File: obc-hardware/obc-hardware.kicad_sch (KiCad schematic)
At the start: 4 parts

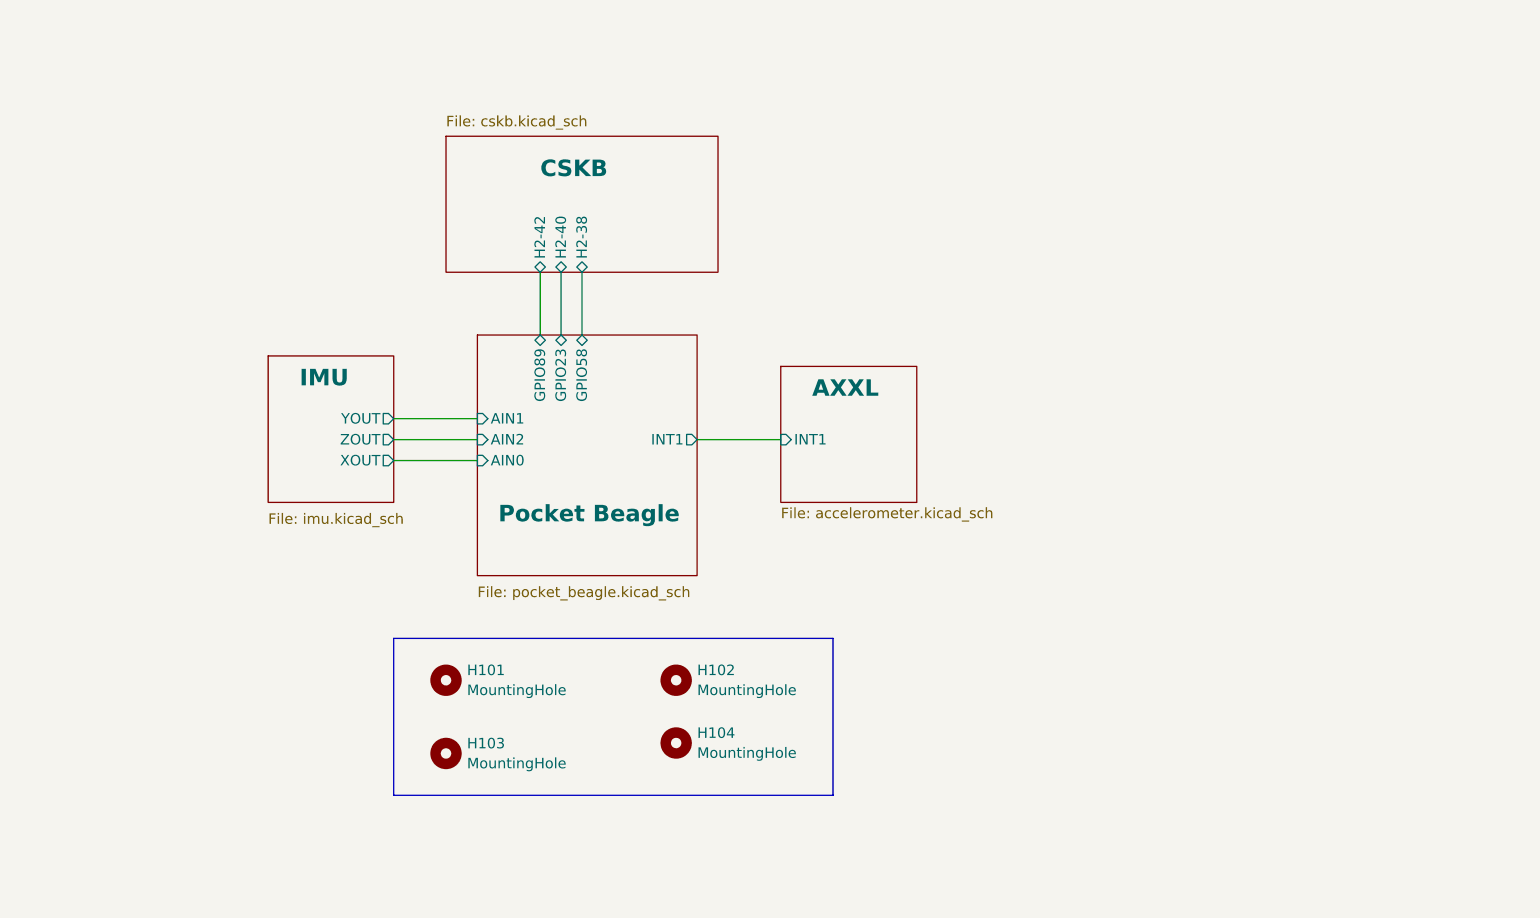
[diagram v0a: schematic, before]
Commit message: added test points
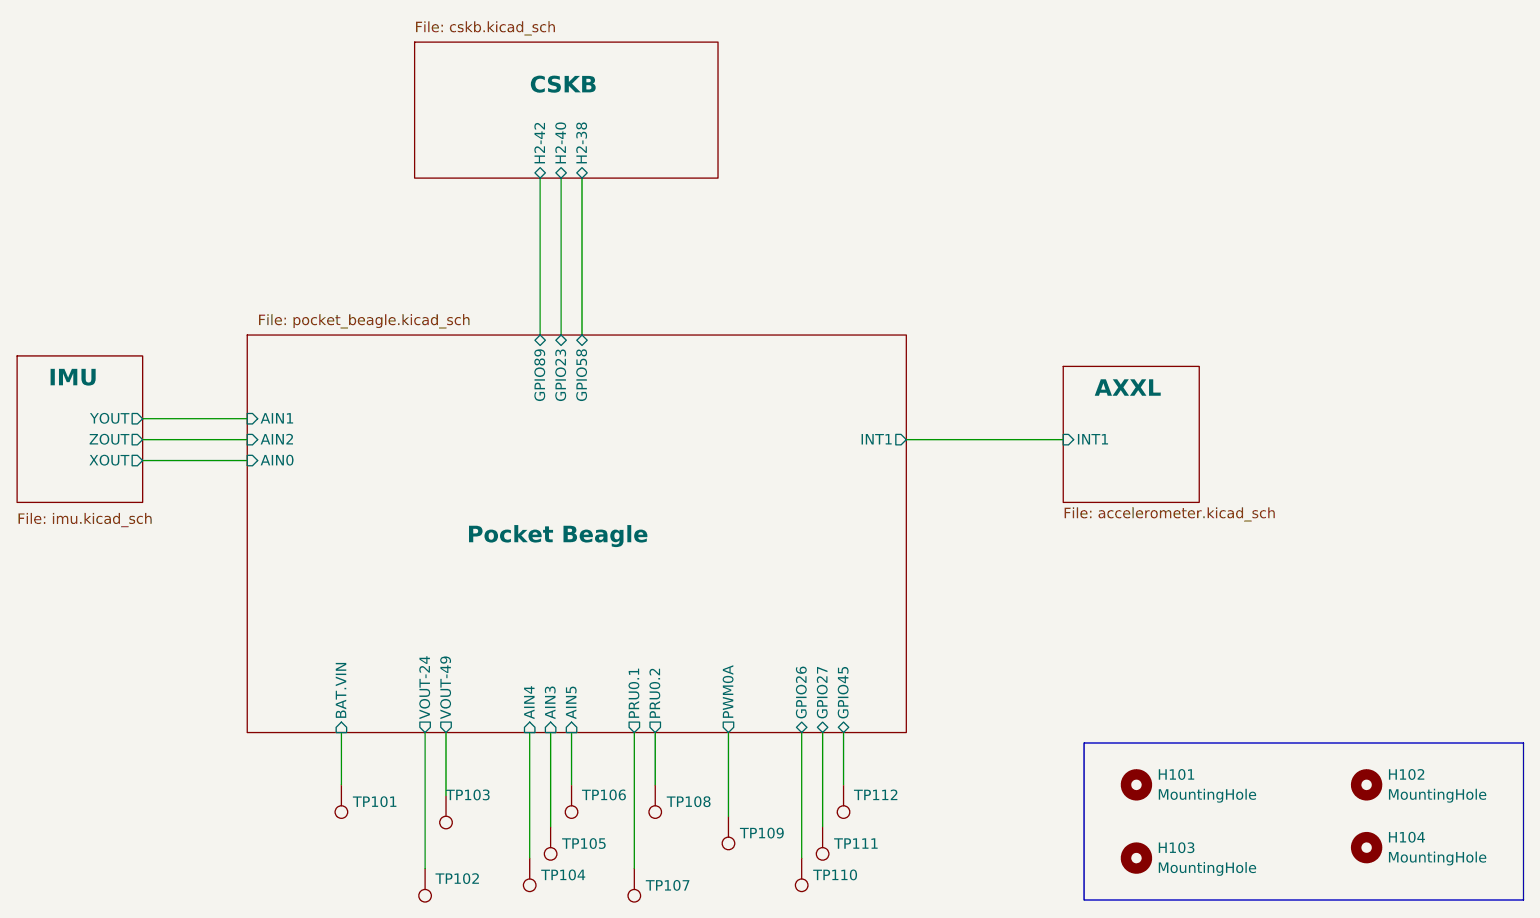
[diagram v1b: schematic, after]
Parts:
- added TP101, TP102, TP103, TP104, TP105, TP106, TP107, TP108, TP109, TP110, TP111, TP112: TestPoint, TestPoint:TestPoint_THTPad_1.0x1.0mm_Drill0.5mm, symbol Connector:TestPoint
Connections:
- new net Pocket Beagle/AIN3: TP105.1
- new net Pocket Beagle/AIN4: TP104.1
- new net Pocket Beagle/AIN5: TP106.1
- new net Pocket Beagle/BAT.VIN: TP101.1
- new net Pocket Beagle/GPIO26: TP110.1
- new net Pocket Beagle/GPIO27: TP111.1
- new net Pocket Beagle/GPIO45: TP112.1
- new net Pocket Beagle/PRU0.1: TP107.1
- new net Pocket Beagle/PRU0.2: TP108.1
- new net Pocket Beagle/PWM0A: TP109.1
- new net Pocket Beagle/VOUT-24: TP102.1
- new net Pocket Beagle/VOUT-49: TP103.1
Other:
- sheet Pocket Beagle ports: added AIN3, AIN4, AIN5, BAT.VIN, GPIO26, GPIO27, GPIO45, PRU0.1, PRU0.2, PWM0A, VOUT-24, VOUT-49; removed none
- moved on the sheet: H101, H102, H103, H104
